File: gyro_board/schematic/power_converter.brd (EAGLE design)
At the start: 64 x 26 mm, 39 parts, among them M1 BSZ097N04LS_G

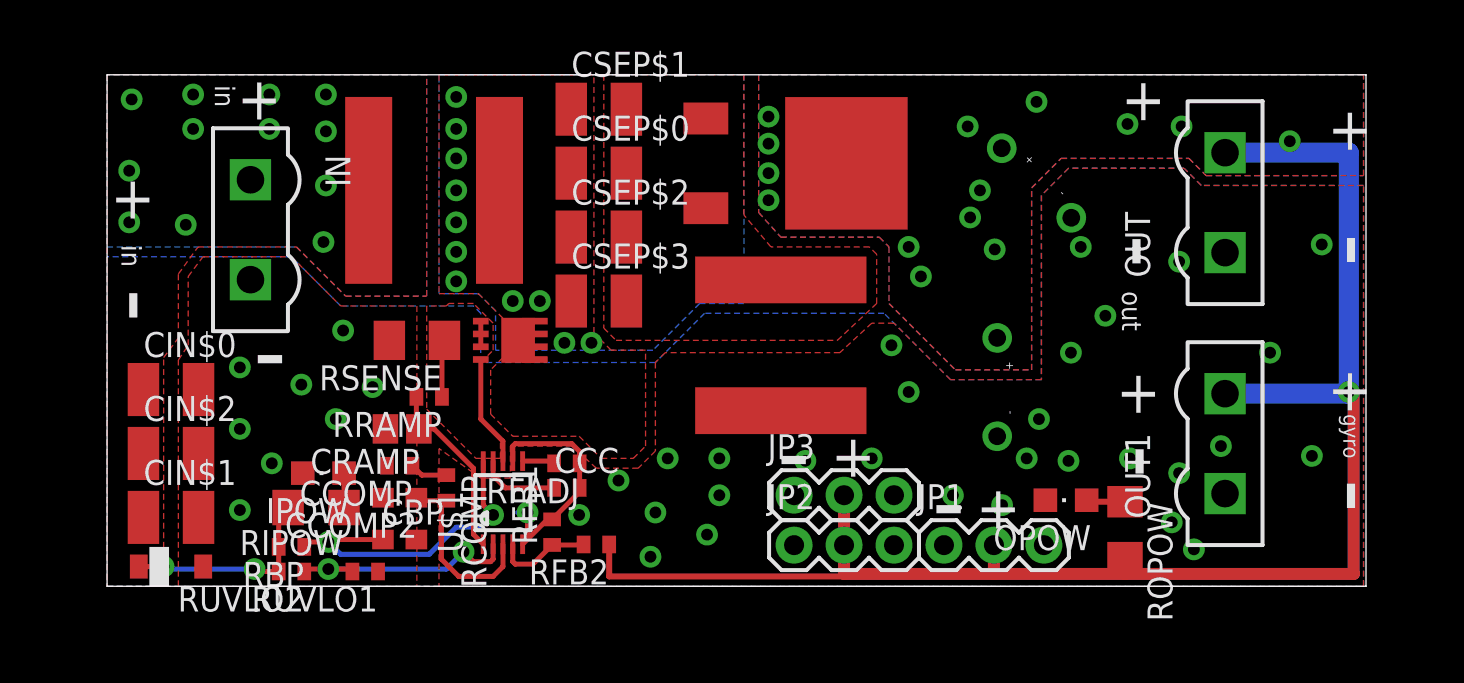
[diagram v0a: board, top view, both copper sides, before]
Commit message: moved the connectors away from the edge
git-svn-id: https://robotics.mvla.net/svn/frc971/2013/trunk/src@4031 f308d9b7-e957-4cde-b6ac-9a88185e7312
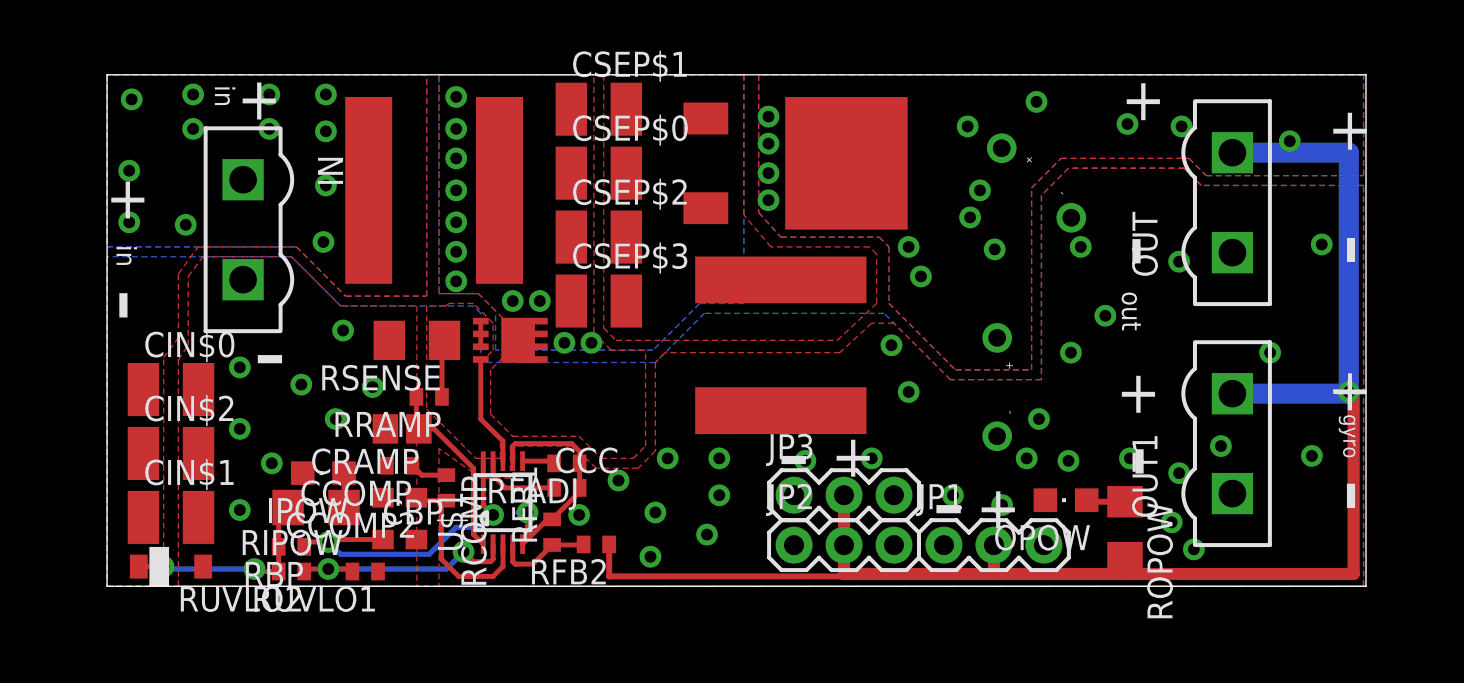
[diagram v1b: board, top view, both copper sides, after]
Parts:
- moved IN 0.38 mm to (4.38, 18.1)
- moved OUT 0.38 mm to (59.8, 19.5)
- moved OUT1 0.38 mm to (59.8, 7.25)
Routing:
- net N$14: track 121.1 -> 120.4 mm
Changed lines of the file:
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@@
 <text x="62.051" y="8.944" size="2.1844" layer="21">+</text>
 <text x="62.051" y="22.194" size="2.1844" layer="21">+</text>
-<text x="0.176" y="18.694" size="2.1844" layer="21">+</text>
-<text x="0.73" y="17.354" size="1" layer="21" font="vector" ratio="10" rot="SR270">in</text>
-<text x="2.763" y="13.431" size="3.81" layer="21" rot="R90">-</text>
+<text x="-0.074" y="18.694" size="2.1844" layer="21">+</text>
+<text x="0.48" y="17.354" size="1" layer="21" font="vector" ratio="10" rot="SR270">in</text>
+<text x="2.263" y="13.431" size="3.81" layer="21" rot="R90">-</text>
 <text x="60.861" y="17.944" size="3.81" layer="21" rot="R270">-</text>
 <text x="60.861" y="5.444" size="3.81" layer="21" rot="R270">-</text>
@@
 <element name="CIN$1" library="resistor" package="C1210" value="C3225X7R1E106M" x="3.25" y="3.5"/>
 <element name="CIN$2" library="resistor" package="C1210" value="C3225X7R1E106M" x="3.25" y="6.75"/>
-<element name="IN" library="custom_parts" package="ELFH0225*" value="POWER_CONNECTORELFH0225*" x="4.75" y="18.125" rot="R270"/>
-<element name="OUT" library="custom_parts" package="ELFH0225*" value="POWER_CONNECTORELFH0225*" x="59.375" y="19.5" rot="R90"/>
+<element name="IN" library="custom_parts" package="ELFH0225*" value="POWER_CONNECTORELFH0225*" x="4.375" y="18.125" rot="R270"/>
+<element name="OUT" library="custom_parts" package="ELFH0225*" value="POWER_CONNECTORELFH0225*" x="59.75" y="19.5" rot="R90"/>
 <element name="DTVS" library="custom_parts" package="SOD-123" value="MMSZ5246BT1G" x="3.25" y="1" rot="R180"/>
 <element name="IPOW" library="led" package="CHIPLED_0805" value="" x="11" y="5.75" rot="R90"/>
@@
 <element name="COUT$0" library="custom_parts" package="RR71C331MDN1" value="" x="45.25" y="10.125" rot="R270"/>
 <element name="COUT$1" library="custom_parts" package="RR71C331MDN1" value="" x="47.25" y="20.5" rot="R315"/>
-<element name="OUT1" library="custom_parts" package="ELFH0225*" value="POWER_CONNECTORELFH0225*" x="59.375" y="7.25" rot="R90"/>
+<element name="OUT1" library="custom_parts" package="ELFH0225*" value="POWER_CONNECTORELFH0225*" x="59.75" y="7.25" rot="R90"/>
 <element name="JP1" library="SparkFun-Connectors" package="1X03" value="" x="42.545" y="2.0895"/>
 <element name="JP2" library="SparkFun-Connectors" package="1X03" value="" x="34.925" y="2.0895"/>
@@
 <wire x1="63.125" y1="9.79" x2="63.125" y2="9.875" width="1.016" layer="16"/>
 <wire x1="63.125" y1="9.875" x2="63.125" y2="22.04" width="1.016" layer="16"/>
-<wire x1="63.125" y1="22.04" x2="56.835" y2="22.04" width="1.016" layer="16"/>
+<wire x1="63.125" y1="22.04" x2="57.21" y2="22.04" width="1.016" layer="16"/>
 <via x="54.625" y="23.375" extent="1-16" drill="0.6"/>
 <via x="51.875" y="23.5" extent="1-16" drill="0.6"/>
@@
 <wire x1="63.375" y1="9.875" x2="63.125" y2="9.875" width="0.3048" layer="1"/>
 <contactref element="OUT1" pad="P$1"/>
-<wire x1="63.125" y1="9.79" x2="56.835" y2="9.79" width="1.016" layer="16"/>
+<wire x1="63.125" y1="9.79" x2="57.21" y2="9.79" width="1.016" layer="16"/>
 <contactref element="JP1" pad="2"/>
 <contactref element="JP2" pad="2"/>
